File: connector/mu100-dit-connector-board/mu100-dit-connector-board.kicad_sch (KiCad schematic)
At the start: 8 parts, among them J1 Conn_01x17_Male, J2 Conn_01x17, J3 Conn_01x10_Female

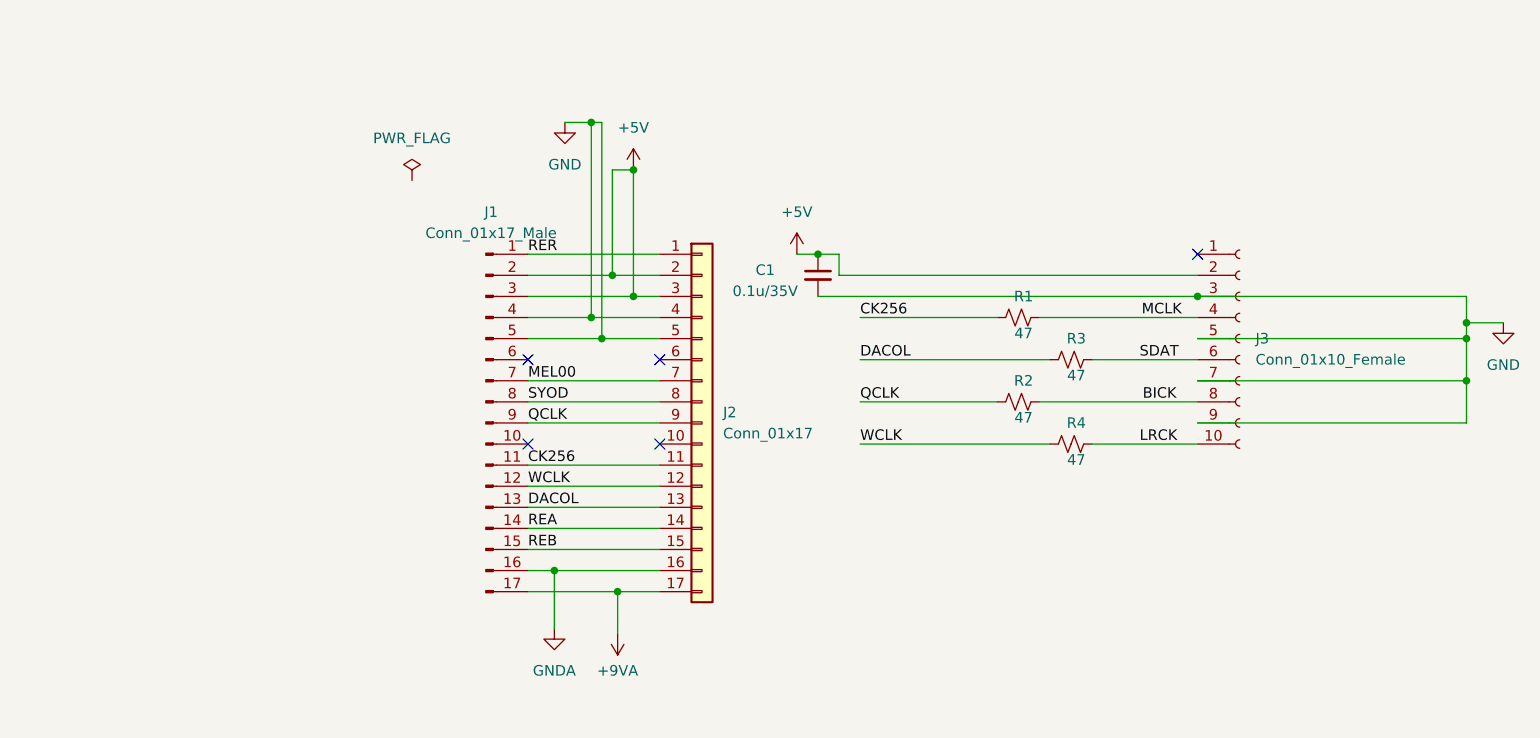
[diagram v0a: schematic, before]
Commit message: finish connector pcb
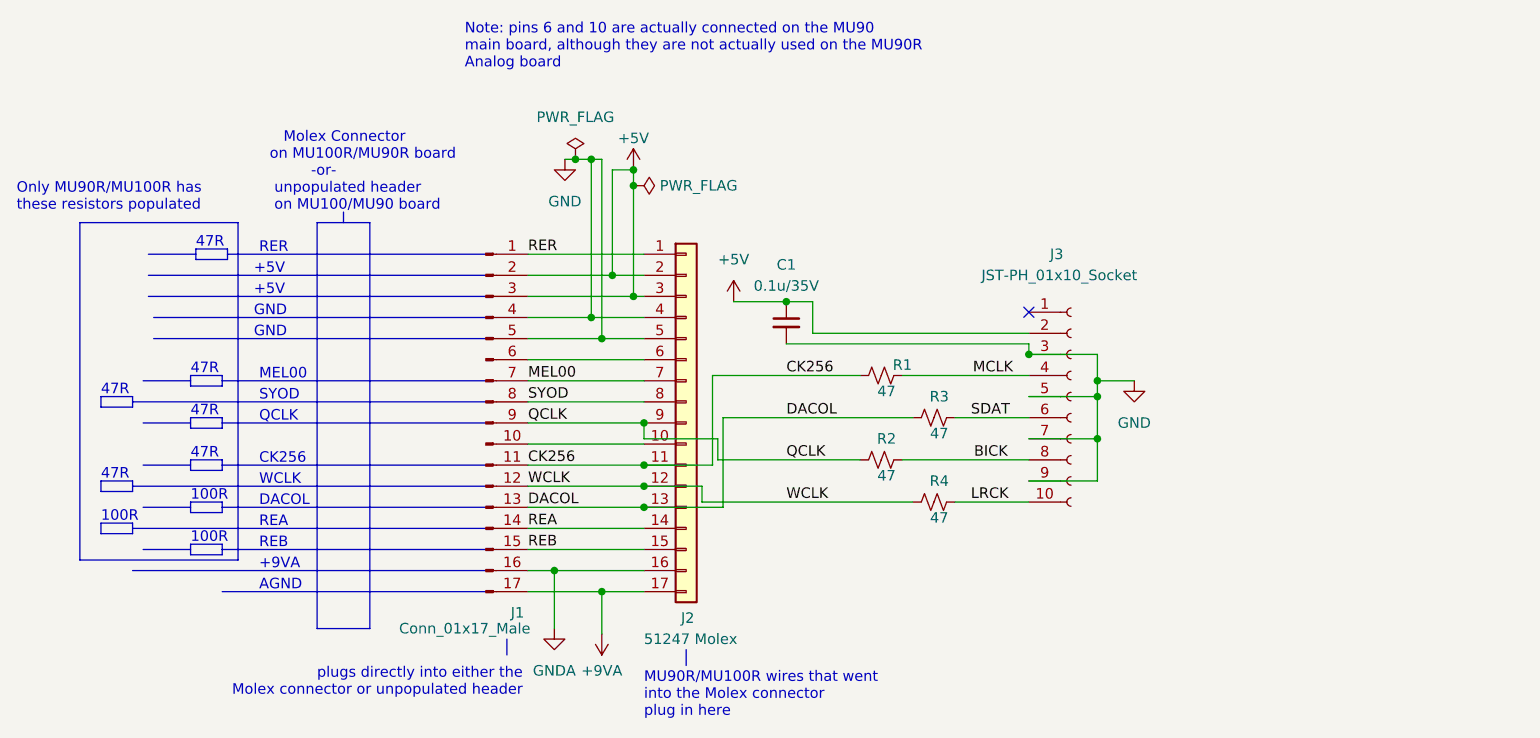
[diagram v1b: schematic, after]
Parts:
- J2: value Conn_01x17 -> 51247 Molex
- J3: value Conn_01x10_Female -> JST-PH_01x10_Socket
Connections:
- net at J2.10 (Pin_10): now also J1.10 (Pin_10)
- net at J2.6 (Pin_6): now also J1.6 (Pin_6)
- no-connect marks 5 -> 1
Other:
- note added: "+5V"
- note added: "+9VA"
- note added: "100R"
- note added: "47R"
- note added: "AGND"
- note added: "CK256"
- note added: "DACOL"
- note added: "GND"
- note added: "MEL00"
- note added: "MU90R/MU100R wires that went into the Molex connector plug in here"
- note added: "Molex Connector on MU100R/MU90R board -or- unpopulated header on MU100/MU90 board"
- note added: "Note: pins 6 and 10 are actually connected on the MU90 main board, although they are not actually used on the MU90R Analog board"
- note added: "Only MU90R/MU100R has these resistors populated"
- note added: "QCLK"
- note added: "REA"
- note added: "REB"
- note added: "RER"
- note added: "SYOD"
- note added: "WCLK"
- note added: "plugs directly into either the Molex connector or unpopulated header"
- moved on the sheet: C1, J2, J3, R1, R2, R3, R4
